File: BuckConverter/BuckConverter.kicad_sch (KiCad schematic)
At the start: 0 parts

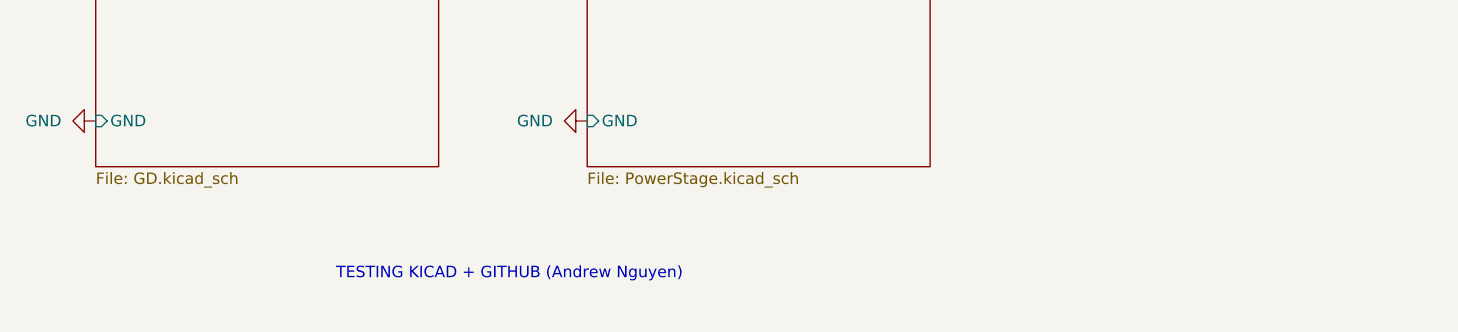
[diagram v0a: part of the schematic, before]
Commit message: Add all footprints
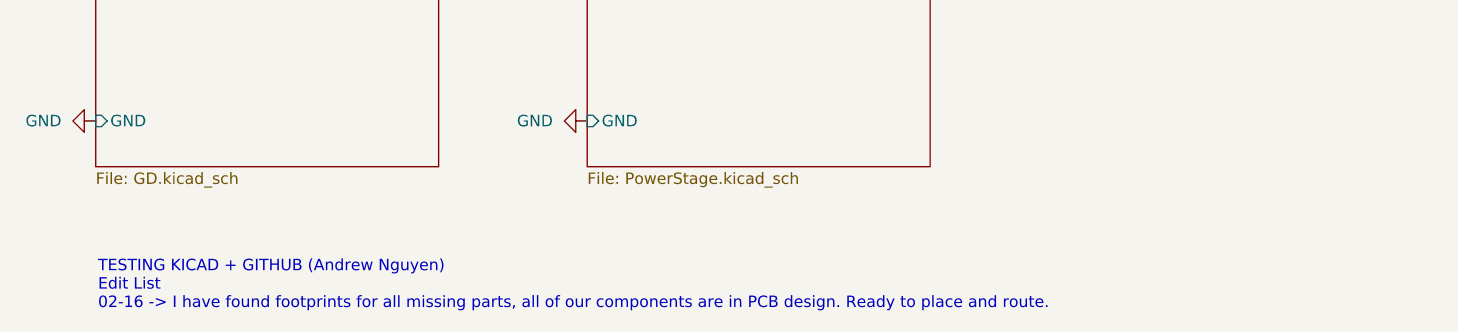
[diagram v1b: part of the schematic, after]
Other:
- note added: "TESTING KICAD + GITHUB (Andrew Nguyen) Edit List 02-16 -> I have found footprints for all missing parts, all of our components are in PCB design. Ready to place and route."
- note removed: "TESTING KICAD + GITHUB (Andrew Nguyen)"
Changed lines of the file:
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@@
 		(rev "v0")
 	)
-	(text "TESTING KICAD + GITHUB (Andrew Nguyen)"
+	(text "TESTING KICAD + GITHUB (Andrew Nguyen)\nEdit List\n02-16 -> I have found footprints for all missing parts, all of our components are in PCB design. Ready to place and route.\n"
 		(exclude_from_sim no)
-		(at 70.104 119.888 0)
+		(at 24.384 121.158 0)
 		(effects
 			(font
 				(size 1.27 1.27)
 			)
+			(justify left)
 		)
 	)

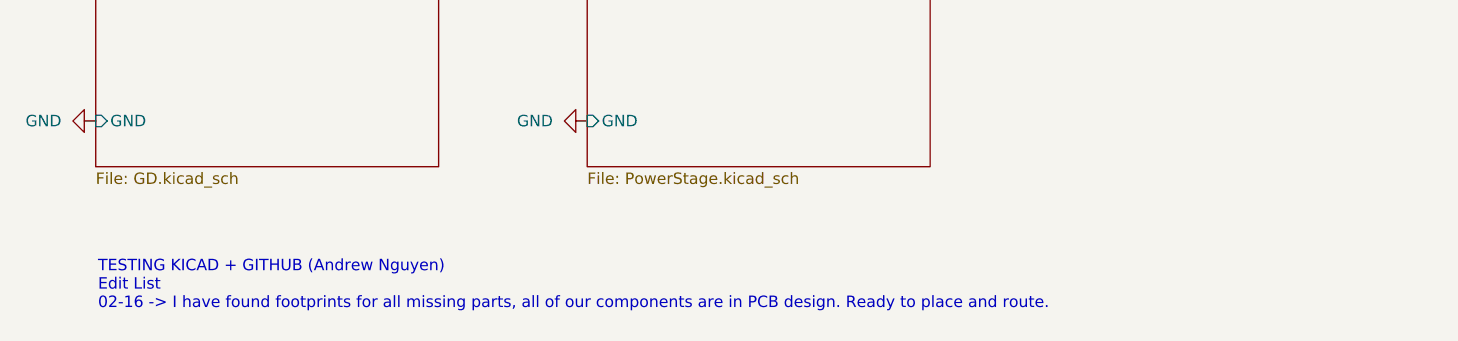
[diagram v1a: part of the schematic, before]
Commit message: PCB Completed
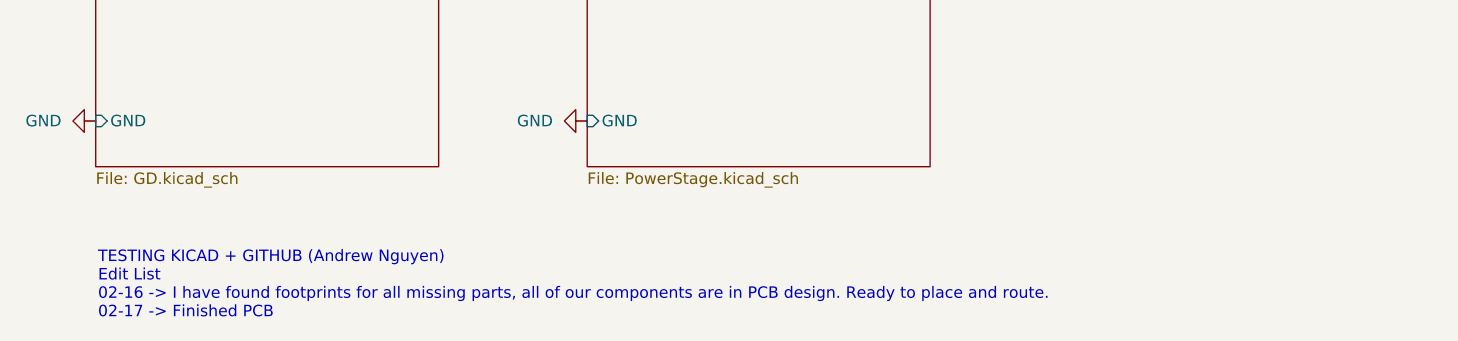
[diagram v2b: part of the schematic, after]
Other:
- note added: "TESTING KICAD + GITHUB (Andrew Nguyen) Edit List 02-16 -> I have found footprints for all missing parts, all of our components are in PCB design. Ready to place and route. 02-17 -> Finished PCB"
- note removed: "TESTING KICAD + GITHUB (Andrew Nguyen) Edit List 02-16 -> I have found footprints for all missing parts, all of our components are in PCB design. Ready to place and route."
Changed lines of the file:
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@@
 		(rev "v0")
 	)
-	(text "TESTING KICAD + GITHUB (Andrew Nguyen)\nEdit List\n02-16 -> I have found footprints for all missing parts, all of our components are in PCB design. Ready to place and route.\n"
+	(text "TESTING KICAD + GITHUB (Andrew Nguyen)\nEdit List\n02-16 -> I have found footprints for all missing parts, all of our components are in PCB design. Ready to place and route.\n02-17 -> Finished PCB"
 		(exclude_from_sim no)
 		(at 24.384 121.158 0)
